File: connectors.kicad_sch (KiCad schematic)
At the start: 11 parts, among them J3 External SPI, J4 JST-PH, J7 USB_C_Receptacle_USB2.0, J8 External UART, J9 External I2C, SW1 Screw Switch Bypass, U2 USBLC6-2SC6

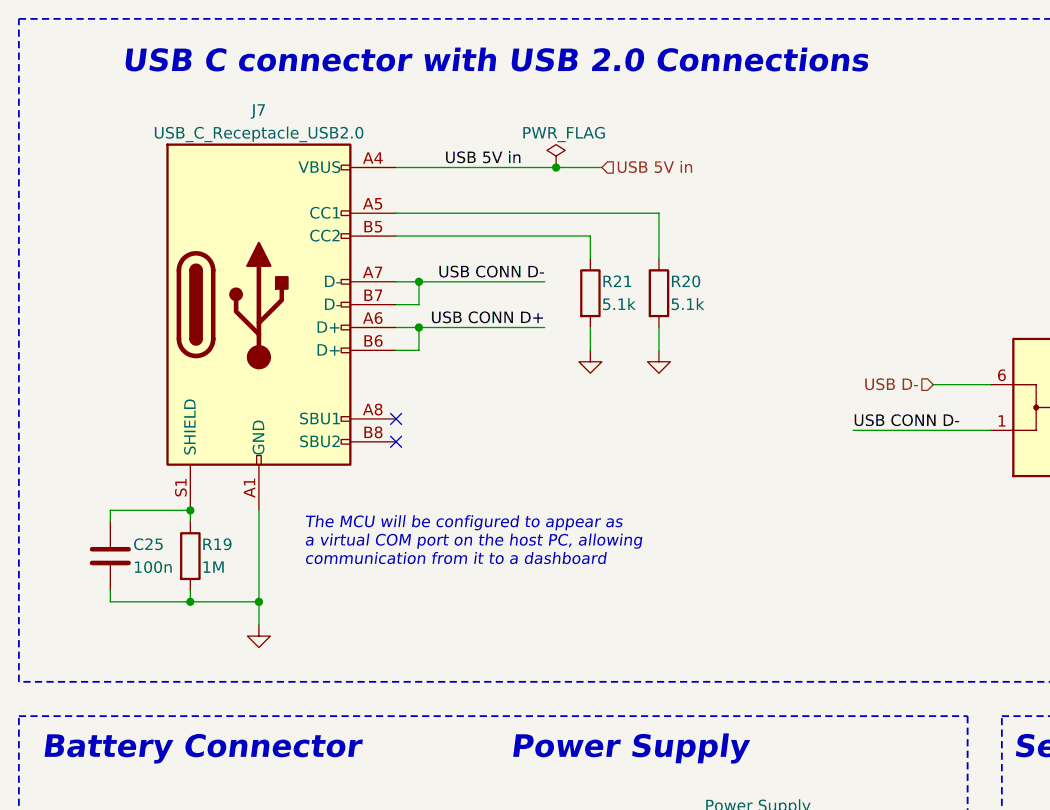
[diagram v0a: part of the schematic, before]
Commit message: Finished preliminary layout of v3
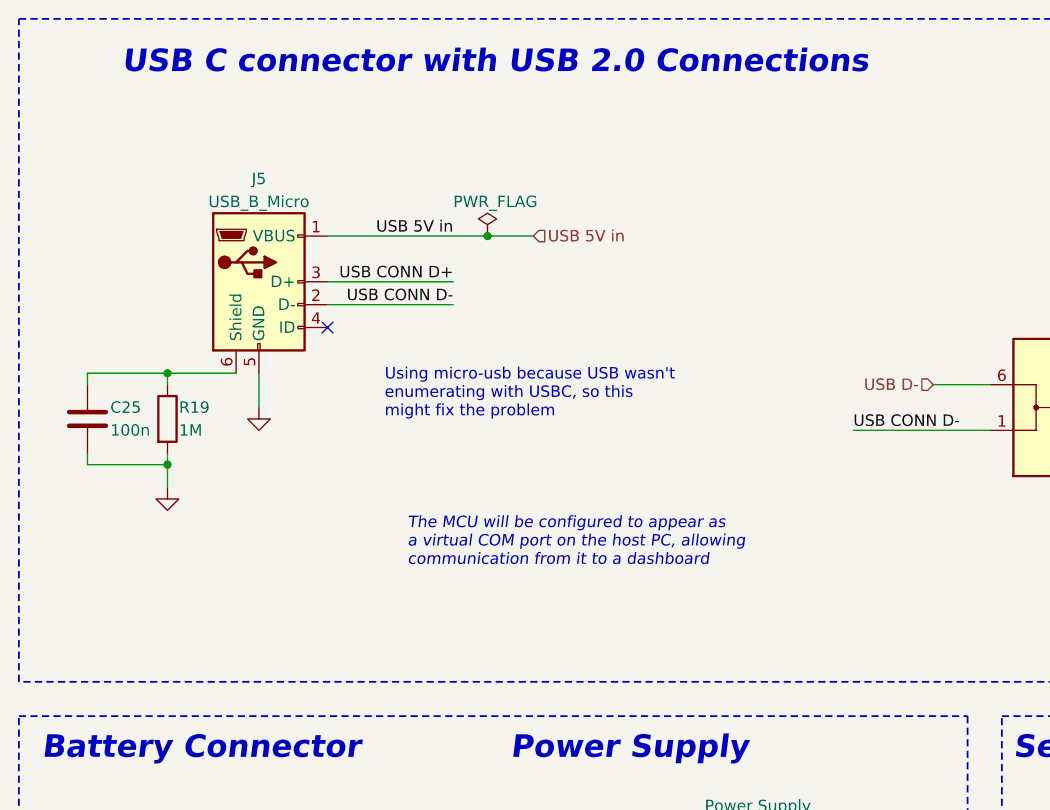
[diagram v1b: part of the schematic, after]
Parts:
- removed J7: USB_C_Receptacle_USB2.0, Connector_USB:USB_C_Receptacle_HRO_TYPE-C-31-M-12, symbol Connector:USB_C_Receptacle_USB2.0
- removed R20, R21: 5.1k, Resistor_SMD:R_0603_1608Metric, symbol Device:R
- added J5: USB_B_Micro, Connector_USB:USB_Micro-B_Amphenol_10118194_Horizontal, symbol Connector:USB_B_Micro
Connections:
- net GND: now also J5.5 (GND)
- net USB 5V in: now also J5.1 (VBUS)
- net USB CONN D+: now also J5.3 (D+)
- net USB CONN D-: now also J5.2 (D-)
- net at C25.1, R19.1: now also J5.6 (Shield)
- no-connect marks 3 -> 2
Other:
- note added: "Using micro-usb because USB wasn't enumerating with USBC, so this might fix the problem"
- moved on the sheet: C25, R19
